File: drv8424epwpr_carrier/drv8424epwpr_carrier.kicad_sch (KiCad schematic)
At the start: 27 parts, among them J1 Input_01x08, J2 Output_01x08, J3 POW_01x02, U1 DRV8424EPWPR, U2 DMP4013LFG-7

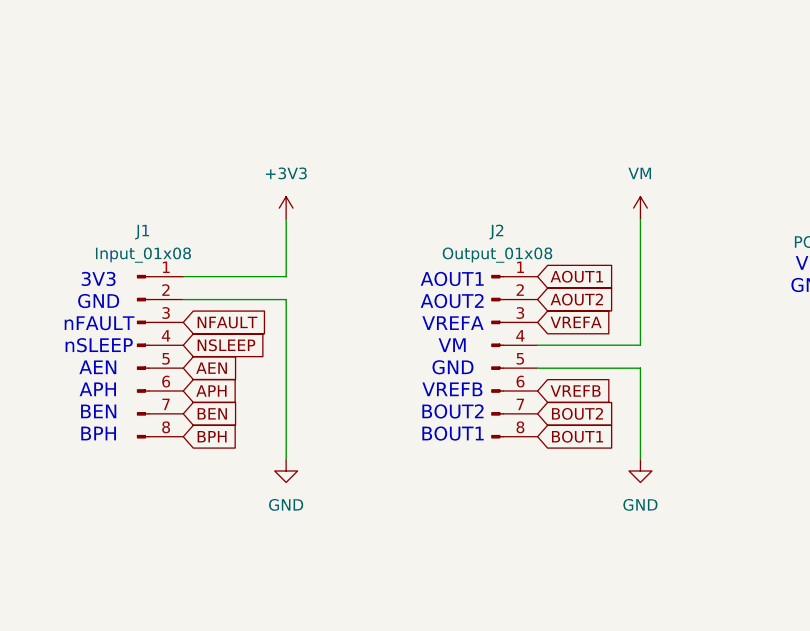
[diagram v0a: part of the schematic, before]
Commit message: update layout
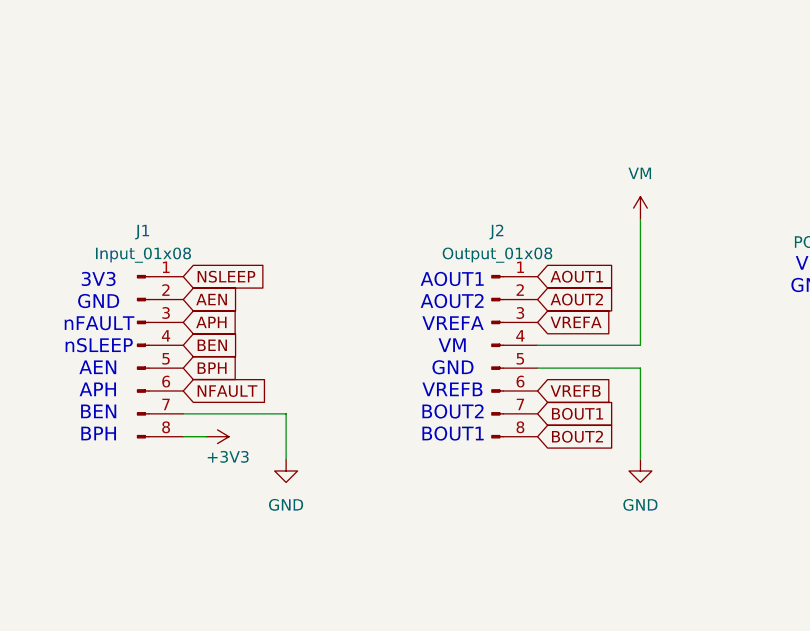
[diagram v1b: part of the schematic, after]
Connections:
- net +3V3: now also J1.8 (Pin_8); no longer J1.1 (Pin_1)
- net AEN: now also J1.2 (Pin_2); no longer J1.5 (Pin_5)
- net APH: now also J1.3 (Pin_3); no longer J1.6 (Pin_6)
- net BEN: now also J1.4 (Pin_4); no longer J1.7 (Pin_7)
- net BOUT1: now also J2.7 (Pin_7); no longer J2.8 (Pin_8)
- net BOUT2: now also J2.8 (Pin_8); no longer J2.7 (Pin_7)
- net BPH: now also J1.5 (Pin_5); no longer J1.8 (Pin_8)
- net GND: now also J1.7 (Pin_7); no longer J1.2 (Pin_2)
- net NFAULT: now also J1.6 (Pin_6); no longer J1.3 (Pin_3)
- net NSLEEP: now also J1.1 (Pin_1); no longer J1.4 (Pin_4)
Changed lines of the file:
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@@
 	(wire
 		(pts
-			(xy 187.96 39.37) (xy 187.96 45.72)
+			(xy 259.08 137.16) (xy 259.08 142.24)
 		)
 		(stroke
@@
 	(wire
 		(pts
-			(xy 259.08 137.16) (xy 259.08 142.24)
+			(xy 93.98 39.37) (xy 105.41 39.37)
 		)
 		(stroke
@@
 	(wire
 		(pts
-			(xy 93.98 39.37) (xy 105.41 39.37)
+			(xy 121.92 118.11) (xy 127 118.11)
 		)
 		(stroke
@@
 	(wire
 		(pts
-			(xy 121.92 118.11) (xy 127 118.11)
+			(xy 114.3 78.74) (xy 124.46 78.74)
 		)
 		(stroke
@@
 	(wire
 		(pts
-			(xy 114.3 78.74) (xy 124.46 78.74)
+			(xy 58.42 109.22) (xy 50.8 109.22)
 		)
 		(stroke
@@
 	(wire
 		(pts
-			(xy 58.42 109.22) (xy 50.8 109.22)
+			(xy 175.26 115.57) (xy 172.72 115.57)
 		)
 		(stroke
@@
 	(wire
 		(pts
-			(xy 175.26 115.57) (xy 172.72 115.57)
+			(xy 68.58 97.79) (xy 72.39 97.79)
 		)
 		(stroke
@@
 	(wire
 		(pts
-			(xy 68.58 97.79) (xy 72.39 97.79)
+			(xy 187.96 60.96) (xy 187.96 66.04)
 		)
 		(stroke
@@
 	(wire
 		(pts
+			(xy 176.53 60.96) (xy 187.96 60.96)
+		)
+		(stroke
+			(width 0)
+			(type default)
+		)
+	)
+	(wire
+		(pts
 			(xy 81.28 73.66) (xy 81.28 78.74)
 		)
@@
 	(wire
 		(pts
-			(xy 187.96 48.26) (xy 187.96 66.04)
-		)
-		(stroke
-			(width 0)
-			(type default)
-		)
-	)
-	(wire
-		(pts
 			(xy 105.41 59.69) (xy 105.41 78.74)
 		)
@@
 	(wire
 		(pts
-			(xy 187.96 45.72) (xy 176.53 45.72)
-		)
-		(stroke
-			(width 0)
-			(type default)
-		)
-	)
-	(wire
-		(pts
 			(xy 259.08 119.38) (xy 259.08 121.92)
 		)
@@
 	(wire
 		(pts
-			(xy 21.59 39.37) (xy 33.02 39.37)
+			(xy 176.53 63.5) (xy 179.07 63.5)
 		)
 		(stroke
@@
 	(wire
 		(pts
-			(xy 74.93 41.91) (xy 74.93 39.37)
+			(xy 21.59 39.37) (xy 33.02 39.37)
 		)
 		(stroke
@@
 	(wire
 		(pts
-			(xy 175.26 118.11) (xy 172.72 118.11)
+			(xy 74.93 41.91) (xy 74.93 39.37)
 		)
 		(stroke
@@
 	(wire
 		(pts
-			(xy 176.53 48.26) (xy 187.96 48.26)
+			(xy 175.26 118.11) (xy 172.72 118.11)
 		)
 		(stroke
@@
 		)
 	)
-	(global_label "BEN"
+	(global_label "BOUT2"
 		(shape input)
-		(at 176.53 60.96 0)
+		(at 215.9 63.5 0)
 		(fields_autoplaced yes)
 		(effects
@@
 		)
 		(property "Intersheetrefs" "${INTERSHEET_REFS}"
-			(at 183.2647 60.96 0)
+			(at 224.9933 63.5 0)
 			(effects
 				(font
@@
 		)
 	)
-	(global_label "BOUT2"
-		(shape input)
-		(at 215.9 60.96 0)
-		(fields_autoplaced yes)
-		(effects
-			(font
-				(size 1.27 1.27)
-			)
-			(justify left)
-		)
-		(property "Intersheetrefs" "${INTERSHEET_REFS}"
-			(at 224.9933 60.96 0)
-			(effects
-				(font
-					(size 1.27 1.27)
-				)
-				(justify left)
-				(hide yes)
-			)
-		)
-	)
 	(global_label "NSLEEP"
 		(shape input)
-		(at 176.53 53.34 0)
+		(at 176.53 45.72 0)
 		(fields_autoplaced yes)
 		(effects
@@
 		)
 		(property "Intersheetrefs" "${INTERSHEET_REFS}"
-			(at 186.6513 53.34 0)
+			(at 186.6513 45.72 0)
 			(effects
 				(font
@@
 		)
 	)
-	(global_label "NFAULT"
+	(global_label "AEN"
 		(shape input)
-		(at 176.53 50.8 0)
+		(at 176.53 48.26 0)
 		(fields_autoplaced yes)
 		(effects
@@
 		)
 		(property "Intersheetrefs" "${INTERSHEET_REFS}"
-			(at 186.3491 50.8 0)
+			(at 183.0833 48.26 0)
 			(effects
 				(font
@@
 	(global_label "APH"
 		(shape input)
+		(at 176.53 50.8 0)
+		(fields_autoplaced yes)
+		(effects
+			(font
+				(size 1.27 1.27)
+			)
+			(justify left)
+		)
+		(property "Intersheetrefs" "${INTERSHEET_REFS}"
+			(at 183.2043 50.8 0)
+			(effects
+				(font
+					(size 1.27 1.27)
+				)
+				(justify left)
+				(hide yes)
+			)
+		)
+	)
+	(global_label "APH"
+		(shape input)
 		(at 175.26 113.03 0)
 		(fields_autoplaced yes)
@@
 		)
 	)
-	(global_label "AEN"
+	(global_label "BEN"
 		(shape input)
-		(at 176.53 55.88 0)
+		(at 176.53 53.34 0)
 		(fields_autoplaced yes)
 		(effects
@@
 		)
 		(property "Intersheetrefs" "${INTERSHEET_REFS}"
-			(at 183.0833 55.88 0)
+			(at 183.2647 53.34 0)
 			(effects
 				(font
@@
 		)
 	)
-	(global_label "VREFA"
+	(global_label "BOUT1"
 		(shape input)
-		(at 172.72 128.27 0)
+		(at 215.9 60.96 0)
 		(fields_autoplaced yes)
 		(effects
@@
 		)
 		(property "Intersheetrefs" "${INTERSHEET_REFS}"
-			(at 181.39 128.27 0)
+			(at 224.9933 60.96 0)
 			(effects
 				(font
@@
 		)
 	)
-	(global_label "VREFA"
+	(global_label "BPH"
 		(shape input)
-		(at 215.9 50.8 0)
+		(at 176.53 55.88 0)
 		(fields_autoplaced yes)
 		(effects
@@
 		)
 		(property "Intersheetrefs" "${INTERSHEET_REFS}"
-			(at 224.57 50.8 0)
+			(at 183.3857 55.88 0)
 			(effects
 				(font
@@
 		)
 	)
-	(global_label "BOUT1"
+	(global_label "VREFA"
 		(shape input)
-		(at 215.9 63.5 0)
+		(at 172.72 128.27 0)
 		(fields_autoplaced yes)
 		(effects
@@
 		)
 		(property "Intersheetrefs" "${INTERSHEET_REFS}"
-			(at 224.9933 63.5 0)
+			(at 181.39 128.27 0)
 			(effects
 				(font
@@
 		)
 	)
-	(global_label "AOUT2"
+	(global_label "NFAULT"
 		(shape input)
-		(at 118.11 113.03 180)
+		(at 176.53 58.42 0)
 		(fields_autoplaced yes)
 		(effects
@@
 				(size 1.27 1.27)
 			)
-			(justify right)
+			(justify left)
 		)
 		(property "Intersheetrefs" "${INTERSHEET_REFS}"
-			(at 109.1981 113.03 0)
+			(at 186.3491 58.42 0)
 			(effects
 				(font
 					(size 1.27 1.27)
 				)
-				(justify right)
+				(justify left)
 				(hide yes)
 			)
 		)
 	)
-	(global_label "BPH"
+	(global_label "VREFA"
 		(shape input)
-		(at 176.53 63.5 0)
+		(at 215.9 50.8 0)
 		(fields_autoplaced yes)
 		(effects
@@
 		)
 		(property "Intersheetrefs" "${INTERSHEET_REFS}"
-			(at 183.3857 63.5 0)
+			(at 224.57 50.8 0)
 			(effects
 				(font
@@
 		)
 	)
-	(global_label "APH"
+	(global_label "AOUT2"
 		(shape input)
-		(at 176.53 58.42 0)
+		(at 118.11 113.03 180)
 		(fields_autoplaced yes)
 		(effects
@@
 				(size 1.27 1.27)
 			)
-			(justify left)
+			(justify right)
 		)
 		(property "Intersheetrefs" "${INTERSHEET_REFS}"
-			(at 183.2043 58.42 0)
+			(at 109.1981 113.03 0)
 			(effects
 				(font
 					(size 1.27 1.27)
 				)
-				(justify left)
+				(justify right)
 				(hide yes)
 			)
@@
 	(symbol
 		(lib_id "power:+3V3")
-		(at 187.96 39.37 0)
+		(at 179.07 63.5 270)
 		(unit 1)
 		(exclude_from_sim no)
@@
 		(on_board yes)
 		(dnp no)
-		(fields_autoplaced yes)
 		(property "Reference" "#PWR013"
-			(at 187.96 43.18 0)
+			(at 175.26 63.5 0)
 			(effects
 				(font
@@
 		)
 		(property "Value" "+3V3"
-			(at 187.96 34.29 0)
+			(at 179.07 65.786 90)
 			(effects
 				(font
 					(size 1.27 1.27)
 				)
+				(justify left)
 			)
 		)
 		(property "Footprint" ""
-			(at 187.96 39.37 0)
+			(at 179.07 63.5 0)
 			(effects
 				(font
@@
 		)
 		(property "Datasheet" ""
-			(at 187.96 39.37 0)
+			(at 179.07 63.5 0)
 			(effects
 				(font
@@
 		)
 		(property "Description" "Power symbol creates a global label with name \"+3V3\""
-			(at 187.96 39.37 0)
+			(at 179.07 63.5 0)
 			(effects
 				(font
